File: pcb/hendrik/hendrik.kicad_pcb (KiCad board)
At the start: 2 copper layers, 58.2 x 53.8 mm, 42 parts, among them IC1 PIC32MK1024MCF064-I_PT, IC2 TPS54331DDAR, IC3 TC1262-3.3VDB, Q1 PN2222A, SW1 SW_Push, SW2 SW_Push

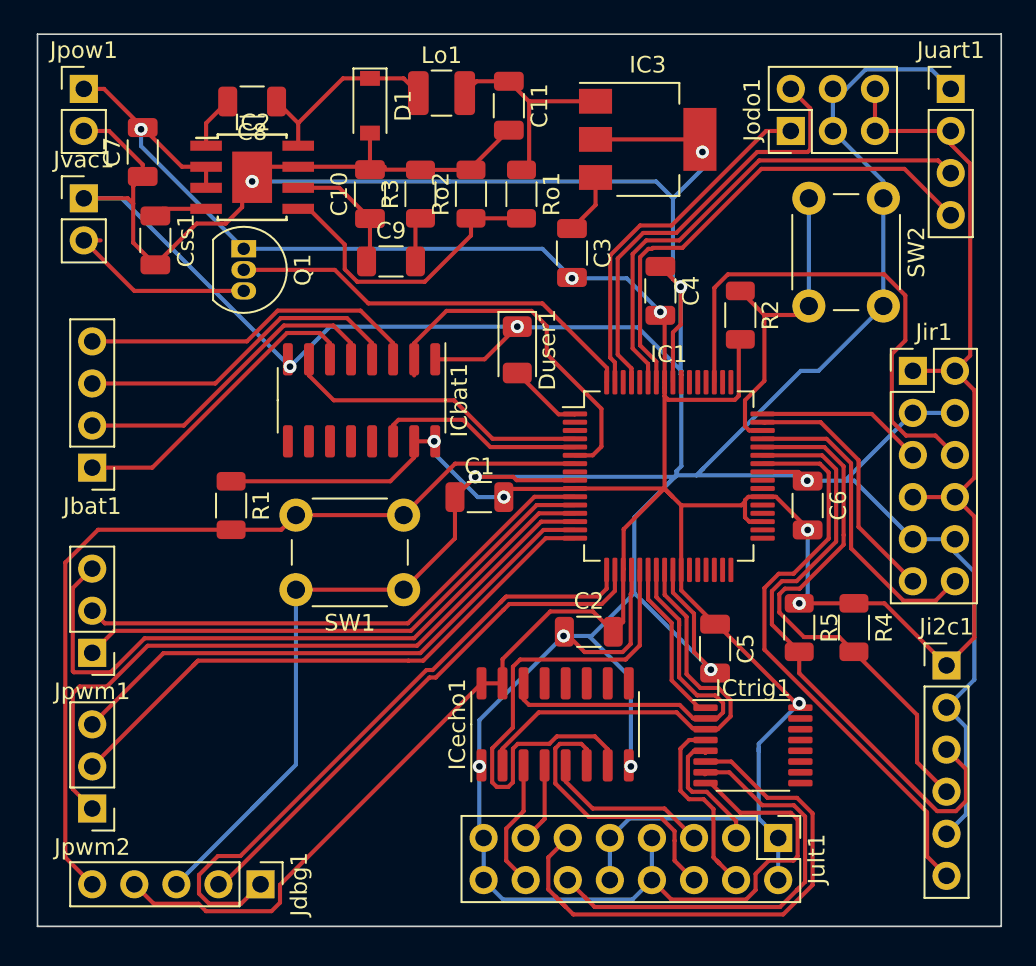
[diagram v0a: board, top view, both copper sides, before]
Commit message: PCB complete
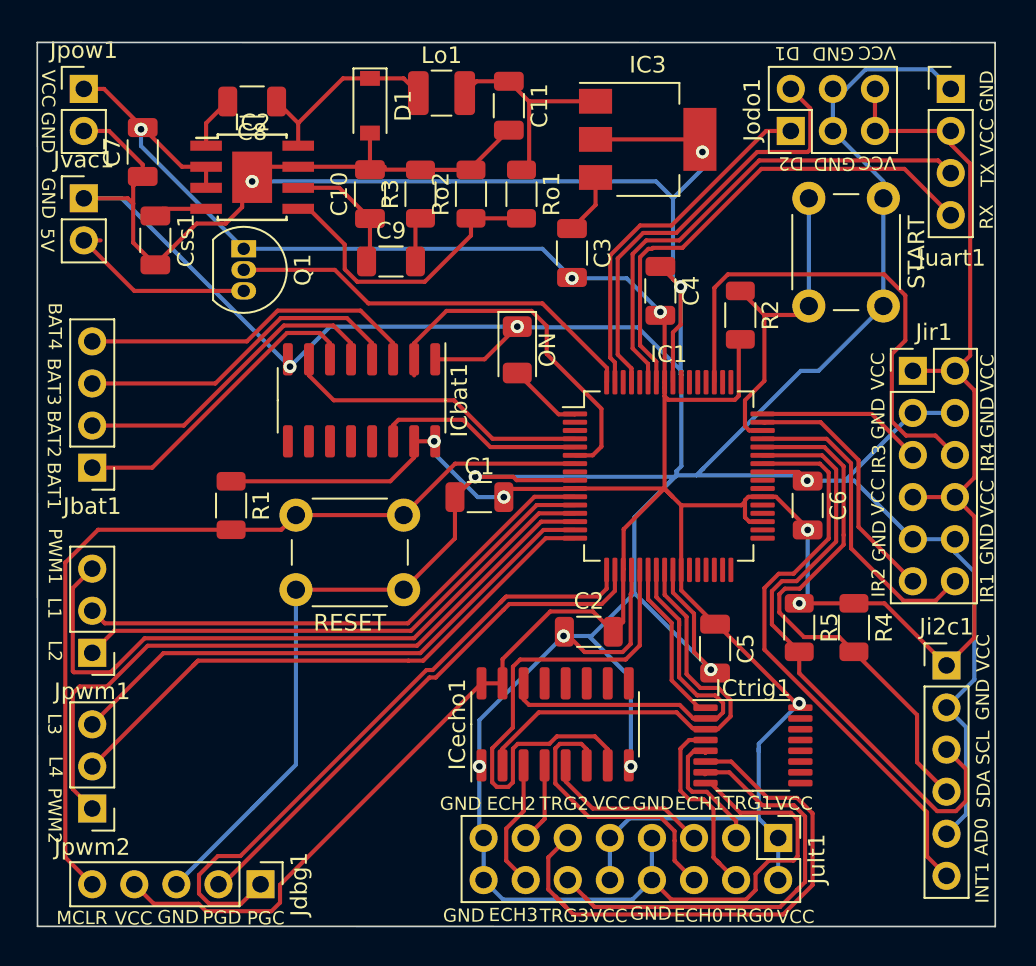
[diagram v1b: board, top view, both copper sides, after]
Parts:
- renumbered Duser1 to ON, SW1 to RESET, SW2 to START
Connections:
- net /AD0 renamed /GND
- net /TX2 renamed /RX1
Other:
- board size 58.2 x 53.8 mm -> 57.8 x 53.4 mm
- board text added: "5V"
- board text added: "AD0"
- board text added: "BAT1"
- board text added: "BAT2"
- board text added: "BAT3"
- board text added: "BAT4"
- board text added: "D1"
- board text added: "D2"
- board text added: "ECH0"
- board text added: "ECH1"
- board text added: "ECH2"
- board text added: "ECH3"
- board text added: "GND"
- board text added: "INT1"
- board text added: "IR1"
- board text added: "IR2"
- board text added: "IR3"
- board text added: "IR4"
- board text added: "L1"
- board text added: "L2"
- board text added: "L3"
- board text added: "L4"
- board text added: "MCLR"
- board text added: "PGC"
- board text added: "PGD"
- board text added: "PWM1"
- board text added: "PWM2"
- board text added: "RX"
- board text added: "SCL"
- board text added: "SDA"
- board text added: "TRG0"
- board text added: "TRG1"
- board text added: "TRG2"
- board text added: "TRG3"
- board text added: "TX"
- board text added: "VCC"
